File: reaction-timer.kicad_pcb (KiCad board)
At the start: 2 copper layers, 48 x 80 mm, 0 parts

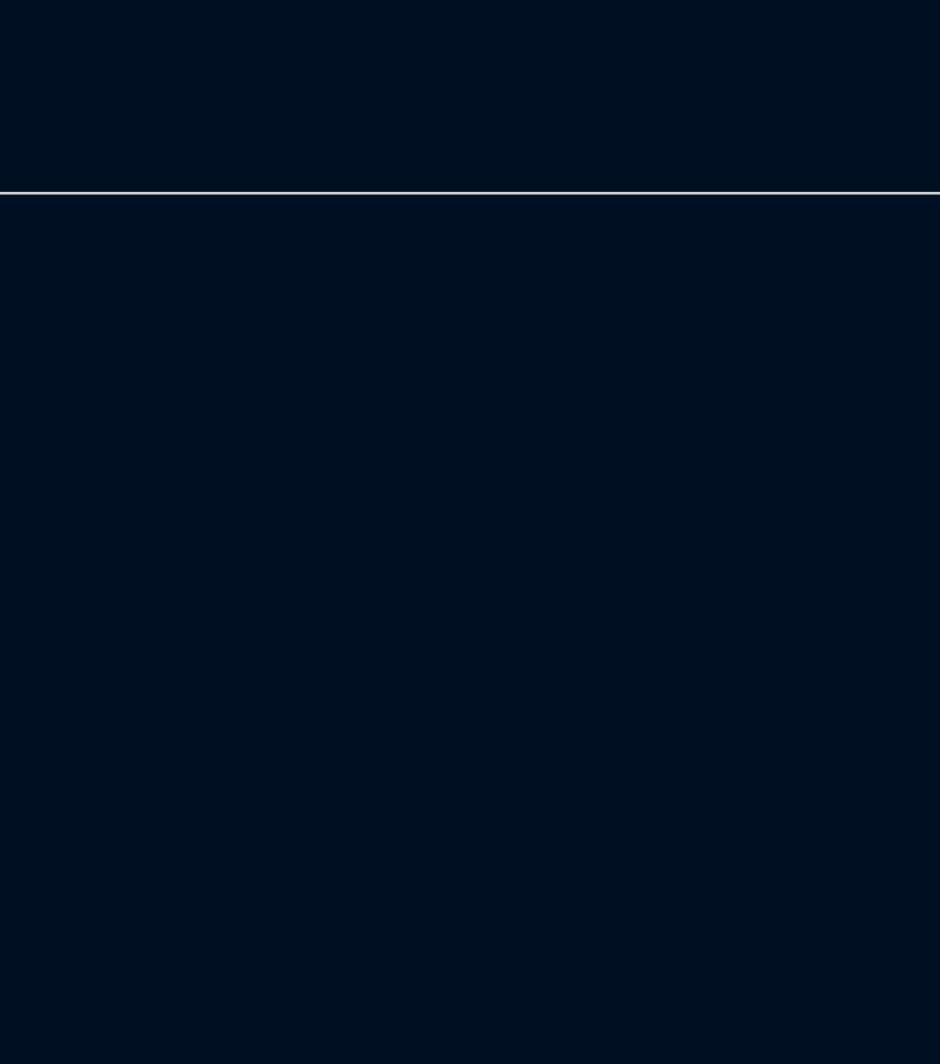
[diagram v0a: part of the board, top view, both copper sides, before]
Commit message: Read netlist
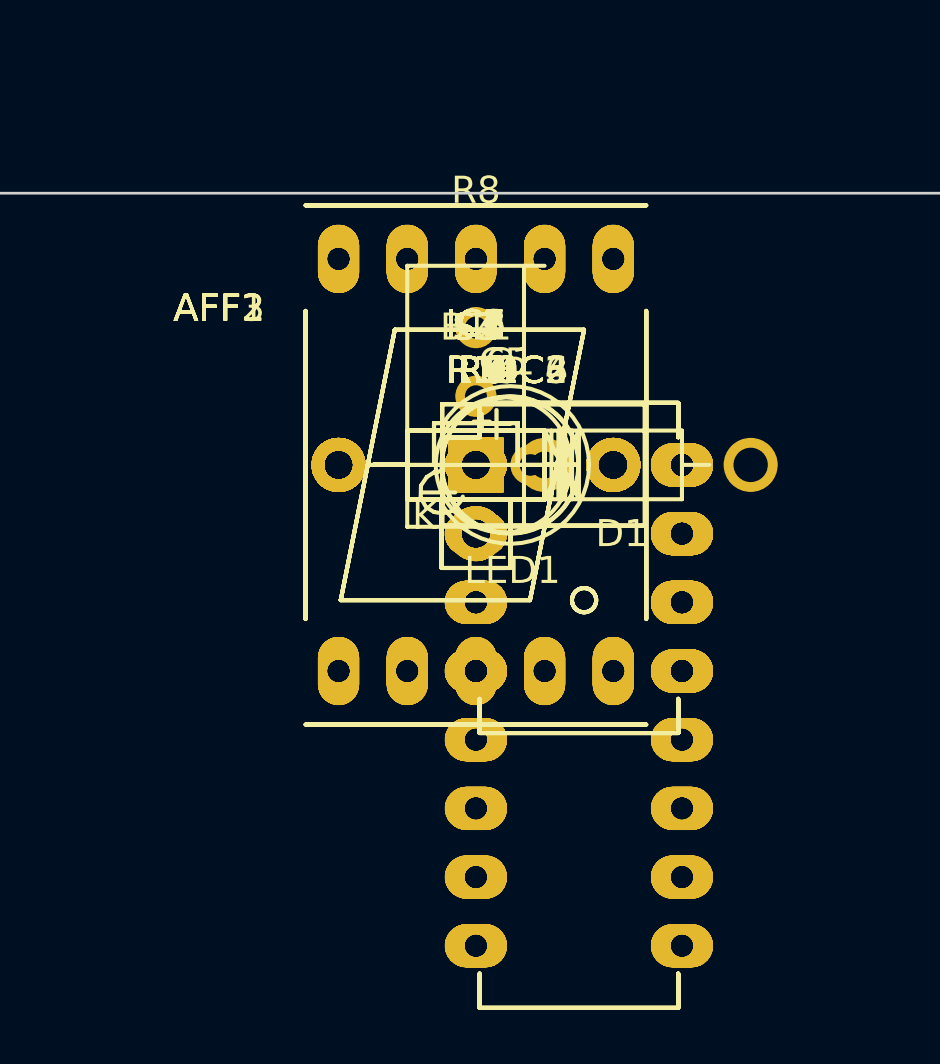
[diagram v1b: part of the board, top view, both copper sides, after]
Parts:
- added AFF1, AFF2, AFF3: LTS-6980HR, Displays_7-Segment:7SegmentLED_LTS6760_LTS6780, F.Cu at (80.0, 150.1)
- added BT1: 9V_Battery, Pin_Headers:Pin_Header_Straight_1x02, F.Cu at (80.0, 150.1)
- added C1: CP, Capacitors_Elko_ThroughHole:Elko_vert_11x5mm_RM2.5, F.Cu at (80.0, 150.1)
- added C2, C3, C4, C6: C, Capacitors_ThroughHole:C_Disc_D7.5_P5, F.Cu at (80.0, 150.1)
- added C5: CP, Capacitors_Elko_ThroughHole:Elko_vert_11x5mm_RM2, F.Cu at (80.0, 150.1)
- added D1: D, Diodes_ThroughHole:Diode_DO-41_SOD81_Horizontal_RM10, F.Cu at (80.0, 150.1)
- added IC1, IC2, IC3: 4026, Housings_DIP:DIP-16_W7.62mm_LongPads, F.Cu at (80.0, 150.1)
- added IC5, IC6, IC7: NE555P, Housings_DIP:DIP-8_W7.62mm_LongPads, F.Cu at (80.0, 150.1)
- added LED1: LED, LEDs:LED-5MM, F.Cu at (80.0, 150.1)
- added R1, R10, R11, R12, R13, R14, R2, R3, R4, R5, R6, R7, R9: R, Resistors_ThroughHole:Resistor_Horizontal_RM10mm, F.Cu at (80.0, 150.1)
- added R8: POT, Potentiometers:Potentiometer_Bourns_3296W_3-8Zoll_Inline_ScrewUp, F.Cu at (80.0, 150.1)
- added S2: SET_TO_ZERO, Pin_Headers:Pin_Header_Straight_1x02, F.Cu at (80.0, 150.1)
- added S3: STOP, Pin_Headers:Pin_Header_Straight_1x02, F.Cu at (80.0, 150.1)
- added S4: START_DELAY, Pin_Headers:Pin_Header_Straight_1x02, F.Cu at (80.0, 150.1)
